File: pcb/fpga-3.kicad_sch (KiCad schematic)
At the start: 6 parts, among them U5 XC7A100T-FGG484, Y1 SiT9365AI-2B2-33E200.000000

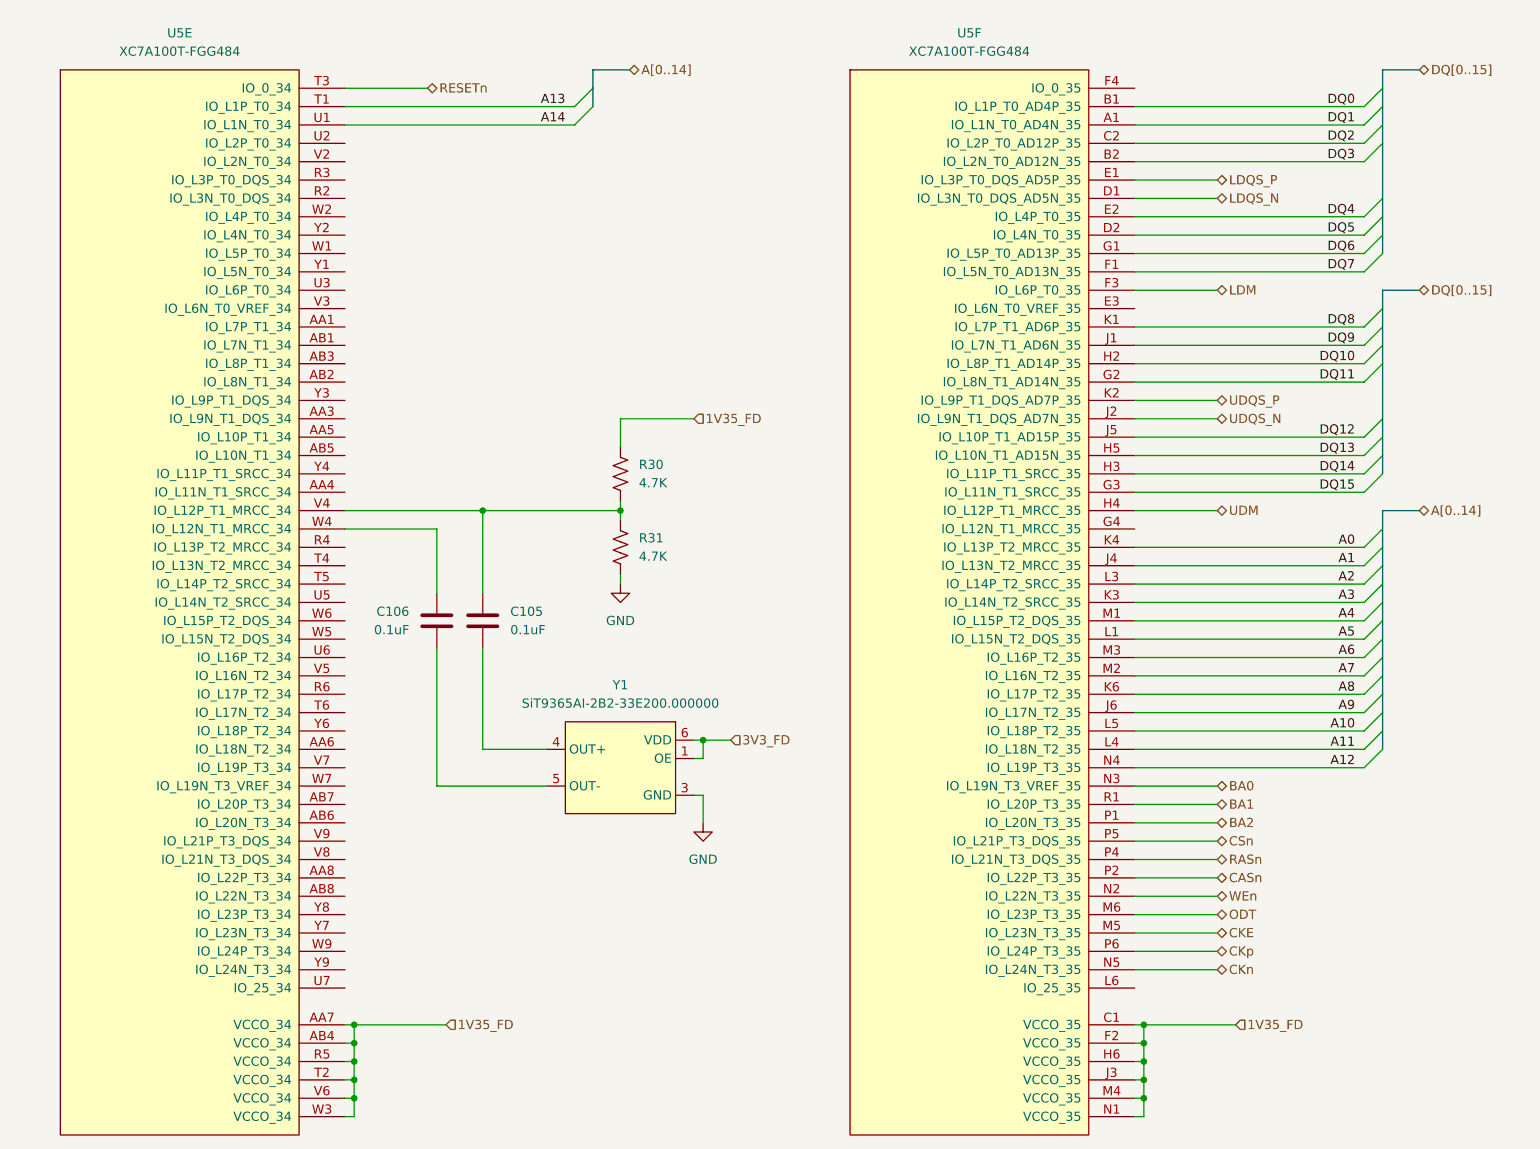
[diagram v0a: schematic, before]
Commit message: power restructuring
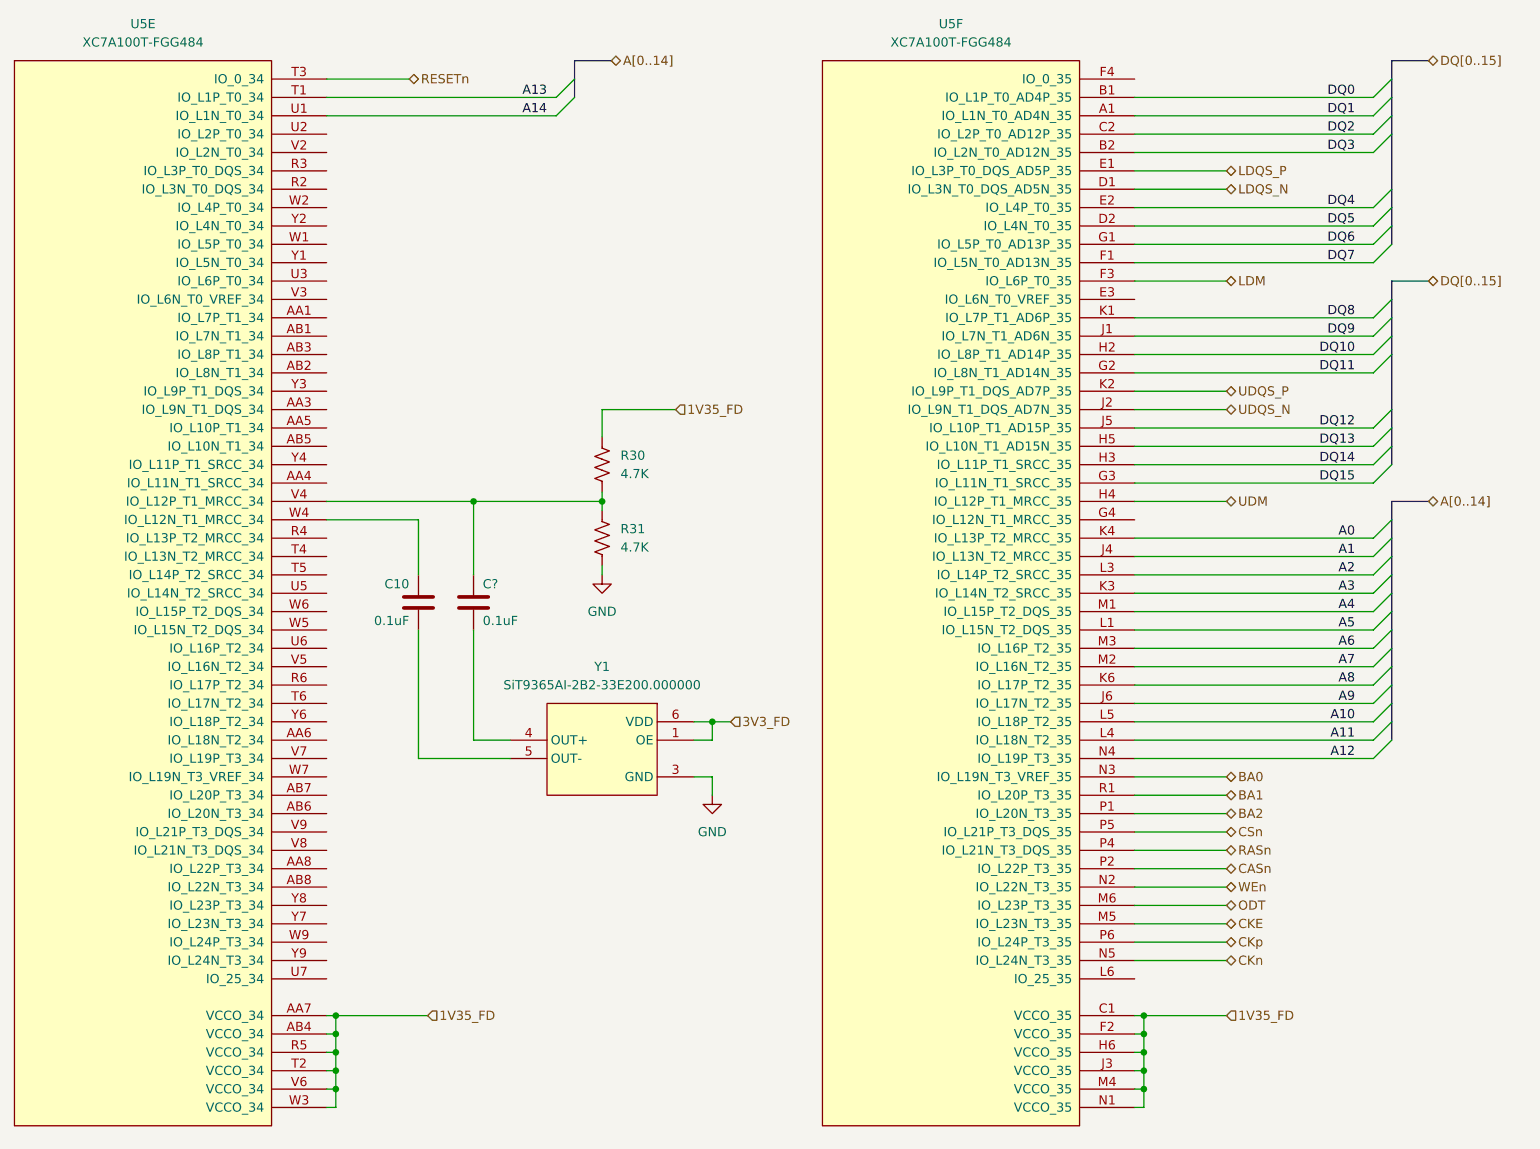
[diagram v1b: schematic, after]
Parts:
- removed C105, C106: 0.1uF, Capacitor_SMD:C_0201_0603Metric, symbol library:C
- removed unit 6 of U5
- added C10, C?: 0.1uF, Capacitor_SMD:C_0402_1005Metric, symbol library:C
- added unit 6 of U5
- U5: symbol FPGA_Xilinx_Artix7:XC7A100T-FGG484 -> library:XC7A100T-FGG484
- Y1: symbol Oscillator:SiT9365xx-xBx-xxE -> library:SiT9365xx-xBx-xxE
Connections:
- net 1V35_FD: now also U5.C1 (VCCO_35), U5.F2 (VCCO_35), U5.H6 (VCCO_35), U5.J3 (VCCO_35), U5.M4 (VCCO_35), U5.N1 (VCCO_35)
- net A0: now also U5.K4 (IO_L13P_T2_MRCC_35)
- net A1: now also U5.J4 (IO_L13N_T2_MRCC_35)
- net A10: now also U5.L5 (IO_L18P_T2_35)
- net A11: now also U5.L4 (IO_L18N_T2_35)
- net A12: now also U5.N4 (IO_L19P_T3_35)
- net A2: now also U5.L3 (IO_L14P_T2_SRCC_35)
- net A3: now also U5.K3 (IO_L14N_T2_SRCC_35)
- net A4: now also U5.M1 (IO_L15P_T2_DQS_35)
- net A5: now also U5.L1 (IO_L15N_T2_DQS_35)
- net A6: now also U5.M3 (IO_L16P_T2_35)
- net A7: now also U5.M2 (IO_L16N_T2_35)
- net A8: now also U5.K6 (IO_L17P_T2_35)
- net A9: now also U5.J6 (IO_L17N_T2_35)
- net BA0: now also U5.N3 (IO_L19N_T3_VREF_35)
- net BA1: now also U5.R1 (IO_L20P_T3_35)
- net BA2: now also U5.P1 (IO_L20N_T3_35)
- net CASn: now also U5.P2 (IO_L22P_T3_35)
- net CKE: now also U5.M5 (IO_L23N_T3_35)
- net CKn: now also U5.N5 (IO_L24N_T3_35)
- net CKp: now also U5.P6 (IO_L24P_T3_35)
- net CSn: now also U5.P5 (IO_L21P_T3_DQS_35)
- net DQ0: now also U5.B1 (IO_L1P_T0_AD4P_35)
- net DQ1: now also U5.A1 (IO_L1N_T0_AD4N_35)
- net DQ10: now also U5.H2 (IO_L8P_T1_AD14P_35)
- net DQ11: now also U5.G2 (IO_L8N_T1_AD14N_35)
- net DQ12: now also U5.J5 (IO_L10P_T1_AD15P_35)
- net DQ13: now also U5.H5 (IO_L10N_T1_AD15N_35)
- net DQ14: now also U5.H3 (IO_L11P_T1_SRCC_35)
- net DQ15: now also U5.G3 (IO_L11N_T1_SRCC_35)
- net DQ2: now also U5.C2 (IO_L2P_T0_AD12P_35)
- net DQ3: now also U5.B2 (IO_L2N_T0_AD12N_35)
- net DQ4: now also U5.E2 (IO_L4P_T0_35)
- net DQ5: now also U5.D2 (IO_L4N_T0_35)
- net DQ6: now also U5.G1 (IO_L5P_T0_AD13P_35)
- net DQ7: now also U5.F1 (IO_L5N_T0_AD13N_35)
- net DQ8: now also U5.K1 (IO_L7P_T1_AD6P_35)
- net DQ9: now also U5.J1 (IO_L7N_T1_AD6N_35)
- net LDM: now also U5.F3 (IO_L6P_T0_35)
- net LDQS_N: now also U5.D1 (IO_L3N_T0_DQS_AD5N_35)
- net LDQS_P: now also U5.E1 (IO_L3P_T0_DQS_AD5P_35)
- net ODT: now also U5.M6 (IO_L23P_T3_35)
- net RASn: now also U5.P4 (IO_L21N_T3_DQS_35)
- net UDM: now also U5.H4 (IO_L12P_T1_MRCC_35)
- net UDQS_N: now also U5.J2 (IO_L9N_T1_DQS_AD7N_35)
- net UDQS_P: now also U5.K2 (IO_L9P_T1_DQS_AD7P_35)
- net WEn: now also U5.N2 (IO_L22N_T3_35)
- net at R30.2, R31.1, U5.V4 (IO_L12P_T1_MRCC_34): now also C?.1
- net at U5.W4 (IO_L12N_T1_MRCC_34): now also C10.1
- net at Y1.4 (OUT+): now also C?.2
- net at Y1.5 (OUT-): now also C10.2
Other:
- moved on the sheet: R30, R31, U5E, Y1
